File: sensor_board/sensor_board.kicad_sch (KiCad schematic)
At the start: 42 parts, among them J1 Conn_02x20_Odd_Even, J2 Conn_Coaxial, J3 Conn_Coaxial, U1 BME280, U2 MPU-6050, U3 NEO-7M-0, U4 RFM95W-868S2, U5 HMC5883L

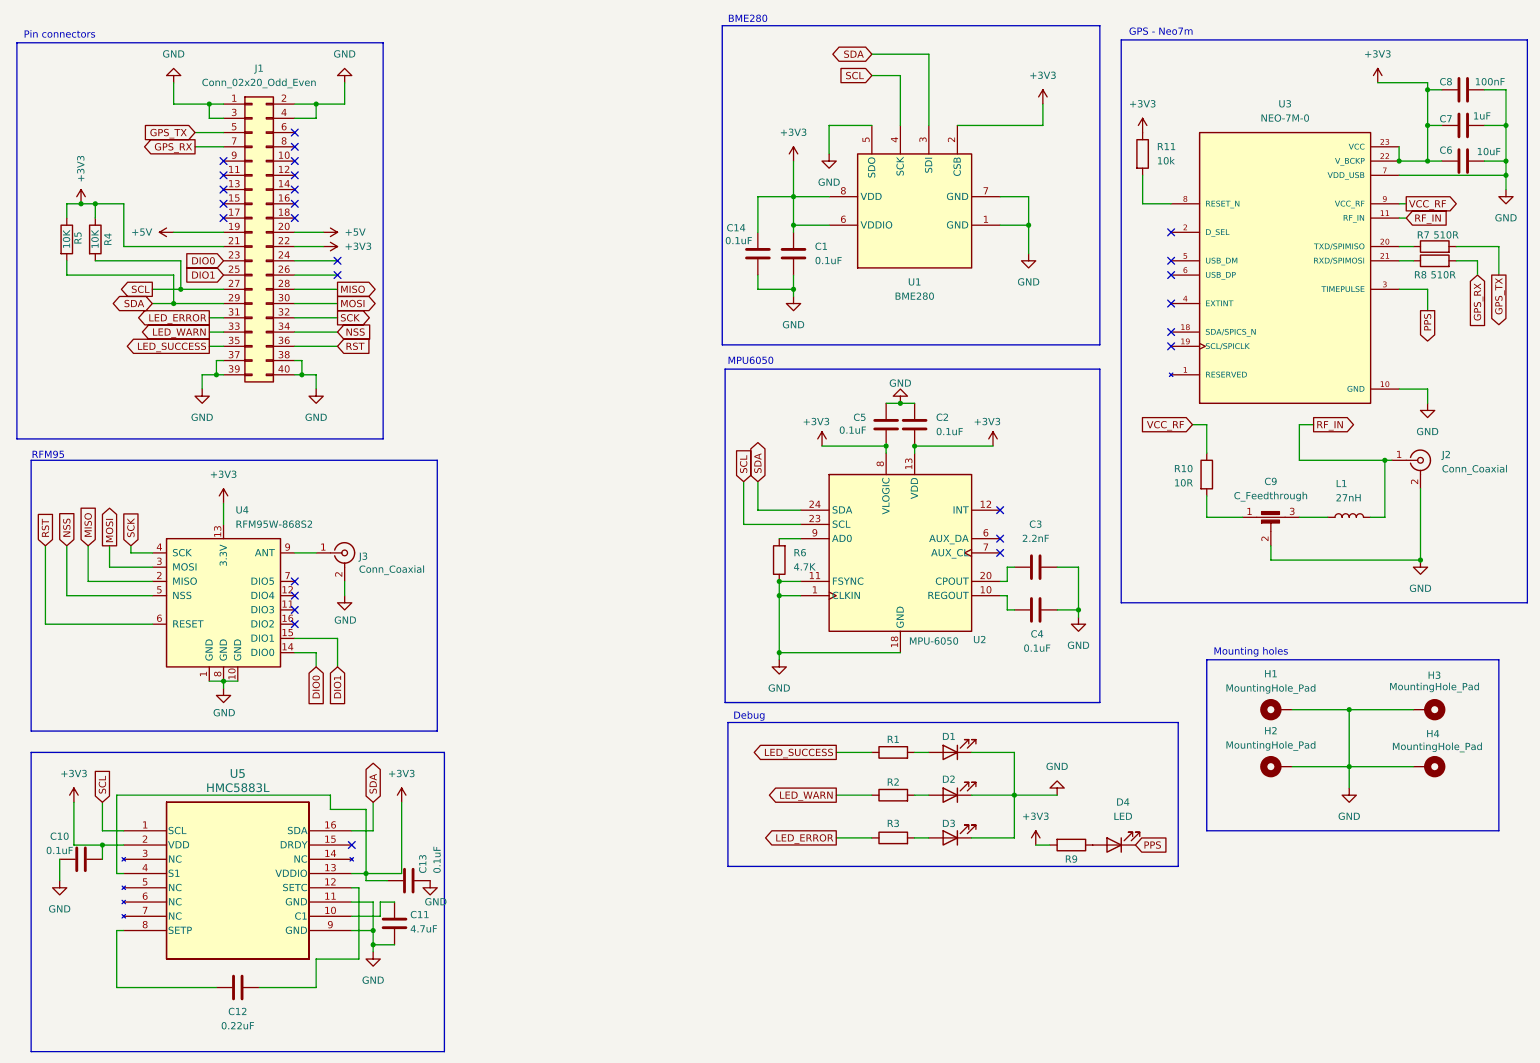
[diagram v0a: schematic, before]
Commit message: completed sensor
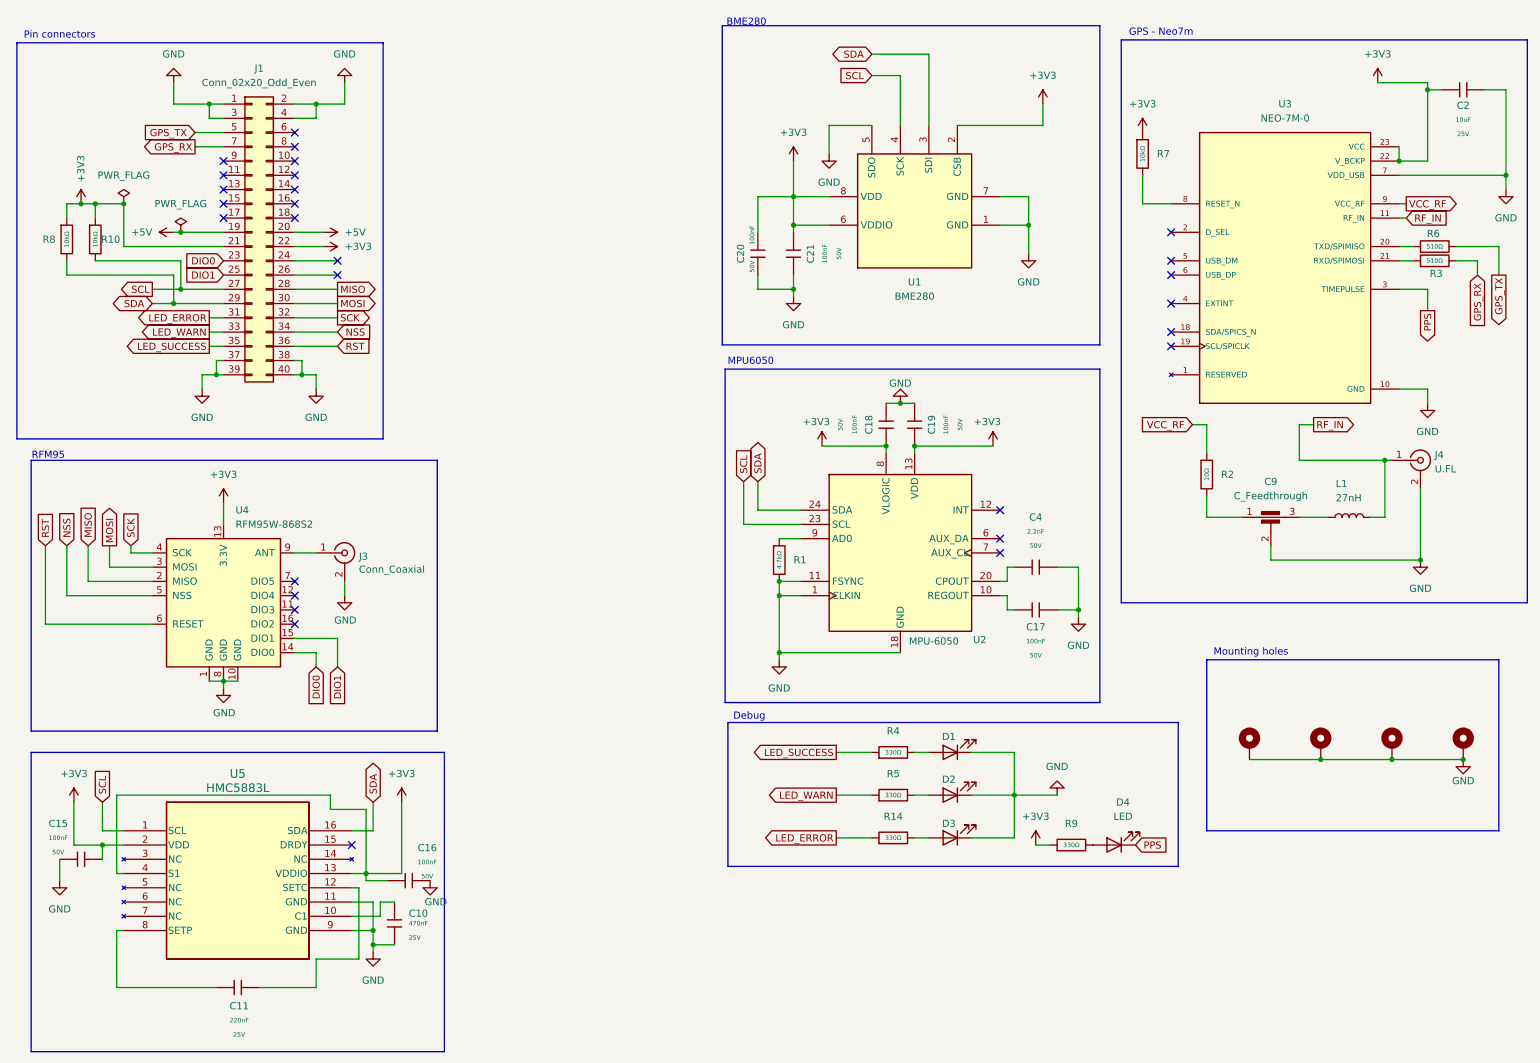
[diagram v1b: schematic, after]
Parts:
- removed C1, C10, C13, C14, C2, C4, C5: 0.1uF, Capacitor_SMD:C_0805_2012Metric, symbol Device:C
- removed C11: 4.7uF, Capacitor_SMD:C_0805_2012Metric, symbol Device:C
- removed C12: 0.22uF, Capacitor_SMD:C_0805_2012Metric, symbol Device:C
- removed C3: 2.2nF, Capacitor_SMD:C_0805_2012Metric, symbol Device:C
- removed C6: 10uF, Capacitor_SMD:C_0805_2012Metric, symbol Device:C
- removed C7: 1uF, Capacitor_SMD:C_0805_2012Metric, symbol Device:C
- removed C8: 100nF, Capacitor_SMD:C_0805_2012Metric, symbol Device:C
- removed H1, H2, H3, H4: MountingHole_Pad, MountingHole:MountingHole_3.2mm_M3_DIN965_Pad, symbol Mechanical:MountingHole_Pad
- removed J2: Conn_Coaxial, Connector_Coaxial:U.FL_Hirose_U.FL-R-SMT-1_Vertical, symbol Connector:Conn_Coaxial
- removed R1, R2, R3: 220, Resistor_SMD:R_0603_1608Metric, symbol Device:R
- removed R10: 10R, Resistor_SMD:R_0603_1608Metric, symbol Device:R
- removed R11: 10k, Resistor_SMD:R_0603_1608Metric, symbol Device:R
- removed R4, R5: 10K, Resistor_SMD:R_0603_1608Metric, symbol Device:R
- removed R6: 4.7K, Resistor_SMD:R_0603_1608Metric, symbol Device:R
- removed R7, R8: 510R, Resistor_SMD:R_0603_1608Metric, symbol Device:R
- removed R9: 220R, Resistor_SMD:R_0603_1608Metric, symbol Device:R
- added C10: 470nF, PCM_JLCPCB:C_0603, symbol PCM_JLCPCB-Capacitors:0603,470nF
- added C11: 220nF, PCM_JLCPCB:C_0603, symbol PCM_JLCPCB-Capacitors:0603,220nF
- added C15, C16, C17, C18, C19, C20, C21: 100nF, PCM_JLCPCB:C_0603, symbol PCM_JLCPCB-Capacitors:0603,100nF
- added C2: 10uF, PCM_JLCPCB:C_0603, symbol PCM_JLCPCB-Capacitors:0603,10uF,(2)
- added C4: 2.2nF, PCM_JLCPCB:C_0603, symbol PCM_JLCPCB-Capacitors:0603,2.2nF
- added J4: U.FL, PCM_JLCPCB:IPEX-SMD_BWIPX-1-001E, symbol PCM_JLCPCB-Extended:RF, Connector, U.FL
- added M1, M2, M3, M4: HOLE, MountingHole:MountingHole_3.2mm_M3_DIN965_Pad, symbol Mechanical:MountingHole_Pad
- added R1: 4.7kΩ, PCM_JLCPCB:R_0603, symbol PCM_JLCPCB-Resistors:0603,4.7kΩ
- added R10, R7, R8: 10kΩ, PCM_JLCPCB:R_0603, symbol PCM_JLCPCB-Resistors:0603,10kΩ
- added R14, R4, R5, R9: 330Ω, PCM_JLCPCB:R_0603, symbol PCM_JLCPCB-Resistors:0603,330Ω
- added R2: 10Ω, PCM_JLCPCB:R_0603, symbol PCM_JLCPCB-Resistors:0603,10Ω
- added R3, R6: 510Ω, PCM_JLCPCB:R_0603, symbol PCM_JLCPCB-Resistors:0603,510Ω
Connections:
- net +3V3: now also C15.2, C16.1, C18.2, C19.1, C2.1, C20.1, C21.2, R10.1, R7.1, R8.1, R9.1
- net GND: now also C10.2, C15.1, C16.2, C17.2, C18.1, C19.2, C2.2, C20.2, C21.1, C4.2, J4.2 (Ext), M1.1, M2.1, M3.1, M4.1, R1.2
- net GPS_RX: now also R3.2
- net GPS_TX: now also R6.2
- net LED_ERROR: now also R14.1
- net LED_SUCCESS: now also R4.1
- net LED_WARN: now also R5.1
- net RF_IN: now also J4.1 (In)
- net SCL: now also R10.2
- net SDA: now also R8.2
- net VCC_RF: now also R2.1
- net at D2.2 (A): now also R5.2
- net at U5.10 (C1): now also C10.1
- net at U5.12 (SETC): now also C11.1
- net at U5.8 (SETP): now also C11.2
- net at U2.10 (REGOUT): now also C17.1
- net at U2.20 (CPOUT): now also C4.1
- net at U2.9 (AD0): now also R1.1
- net at U3.8 (RESET_N): now also R7.2
- net at D3.2 (A): now also R14.2
- net at C9.1: now also R2.2
- net at U3.20 (TXD/SPIMISO): now also R6.1
- net at U3.21 (RXD/SPIMOSI): now also R3.1
- net at D1.2 (A): now also R4.2
- net at D4.2 (A): now also R9.2
